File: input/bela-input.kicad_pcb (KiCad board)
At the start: 2 copper layers, 114.3 x 31.8 mm, 67 parts, among them P1 MTA-156-4, P2 in_mod, P3 out_bela, U1 TL074, U2 TL074, U3 TL071

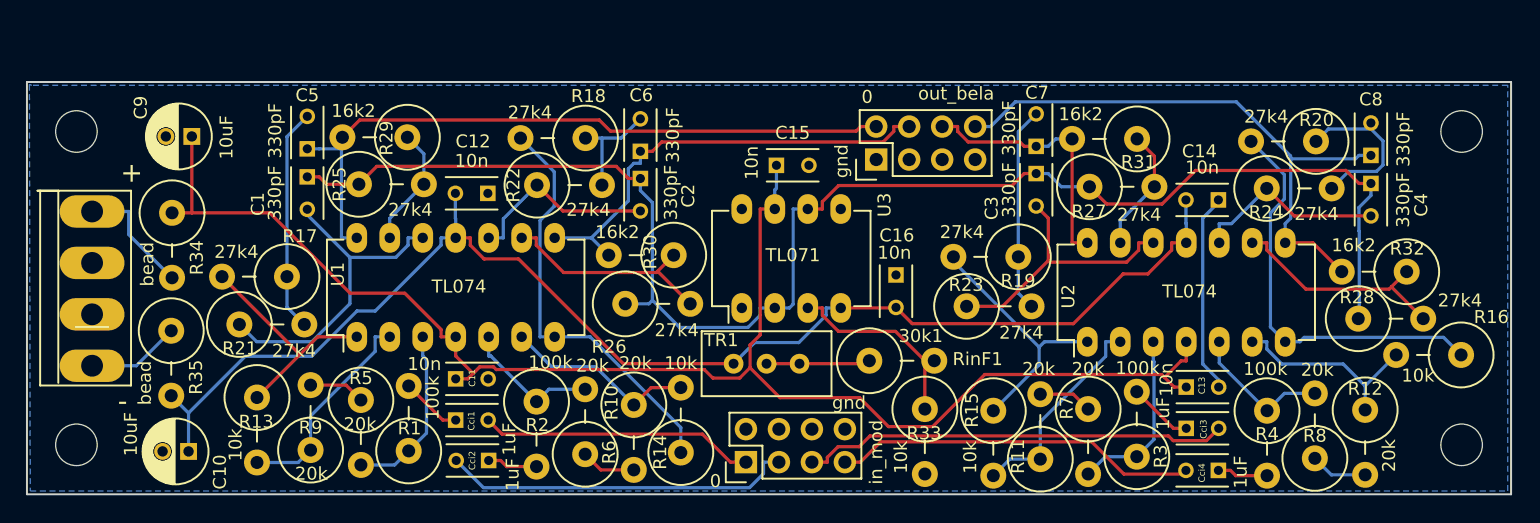
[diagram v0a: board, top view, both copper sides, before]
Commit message: relayout of input
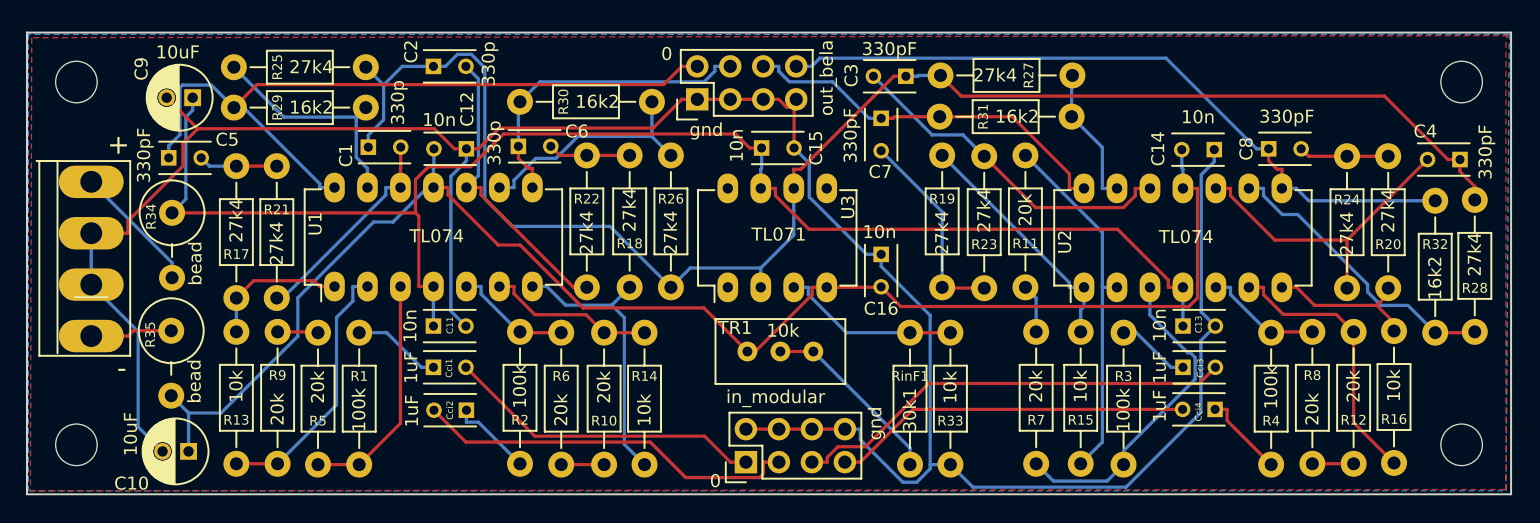
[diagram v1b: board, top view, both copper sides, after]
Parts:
- C1, C2, C6: value 330pF -> 330p
- P2: value in_mod -> in_modular
- R1, R10, R11, R12, R13, R14, R15, R16, R17, R18, R19, R2, R20, R21, R22, R23, R24, R25, R26, R27, R28, R29, R3, R30, R31, R32, R33, R4, R5, R6, R7, R8, R9, RinF1: footprint Resistors_ThroughHole:Resistor_Vertical_RM5mm -> xnorman:Resistor_Horizontal_RM10mm-xnorman
- R34, R35: footprint Resistors_ThroughHole:Resistor_Vertical_RM5mm -> xnorman:Resistor_Vertical_RM5mm-xnor
- TR1: value TRIM -> 10k
- moved R11 20.9 mm to (153.1, 75.5), turned to 270 degrees
- moved C2 18.1 mm to (107.5, 68.6), turned to 0 degrees
- moved R27 16.4 mm to (146.6, 69.3)
- moved P3 14.5 mm to (127.8, 71.2)
- moved C3 12.5 mm to (143.9, 69.4), turned to 180 degrees
- moved C7 12.1 mm to (142.0, 72.6), turned to 270 degrees
- moved R30 11.8 mm to (124.3, 71.4)
- moved R23 11.6 mm to (149.9, 75.6), turned to 270 degrees
- moved R28 11.2 mm to (187.7, 78.9), turned to 270 degrees
- moved R15 10.9 mm to (157.4, 89.1)
- moved C5 10.7 mm to (87.1, 75.7), turned to 0 degrees
- moved C6 9.41 mm to (114.0, 74.8), turned to 0 degrees
- moved R7 9.34 mm to (153.9, 89.1)
- moved R25 9.23 mm to (102.3, 68.7), turned to 180 degrees
- moved R17 8.62 mm to (92.3, 76.3), turned to 270 degrees
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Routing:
- net GND: track 15.4 -> 194.5 mm
- net Net-(R16-Pad1): track 31.7 -> 12.1 mm
- net VSS: track 104.2 -> 116.1 mm
- net Net-(R11-Pad1): track 16.4 -> 28.0 mm
- net Net-(R3-Pad1): track 13.7 -> 25.3 mm
- net Net-(C5-Pad2): track 17.2 -> 6.08 mm
- net Net-(R14-Pad1): track 32.5 -> 22.0 mm
- net bela_ain3: track 45.2 -> 55.4 mm
- net bela_ain1: track 35.0 -> 24.8 mm
- net Net-(C4-Pad2): track 15.2 -> 24.5 mm
- net bela_ain2: track 20.2 -> 29.6 mm
- net Net-(C1-Pad2): track 25.5 -> 16.5 mm
- net Net-(R25-Pad2): track 9.36 -> 17.8 mm
- net Net-(C2-Pad2): track 15.1 -> 22.9 mm
- net Net-(R13-Pad1): track 18.1 -> 10.9 mm
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- added copper zone on F.Cu, net GND
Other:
- board size 114.3 x 31.8 mm -> 114.3 x 35.6 mm
- board text added: "modular to bela analog"
- board text removed: "mod to bela analog"
